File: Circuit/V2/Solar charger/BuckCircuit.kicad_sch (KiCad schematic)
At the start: 2 parts

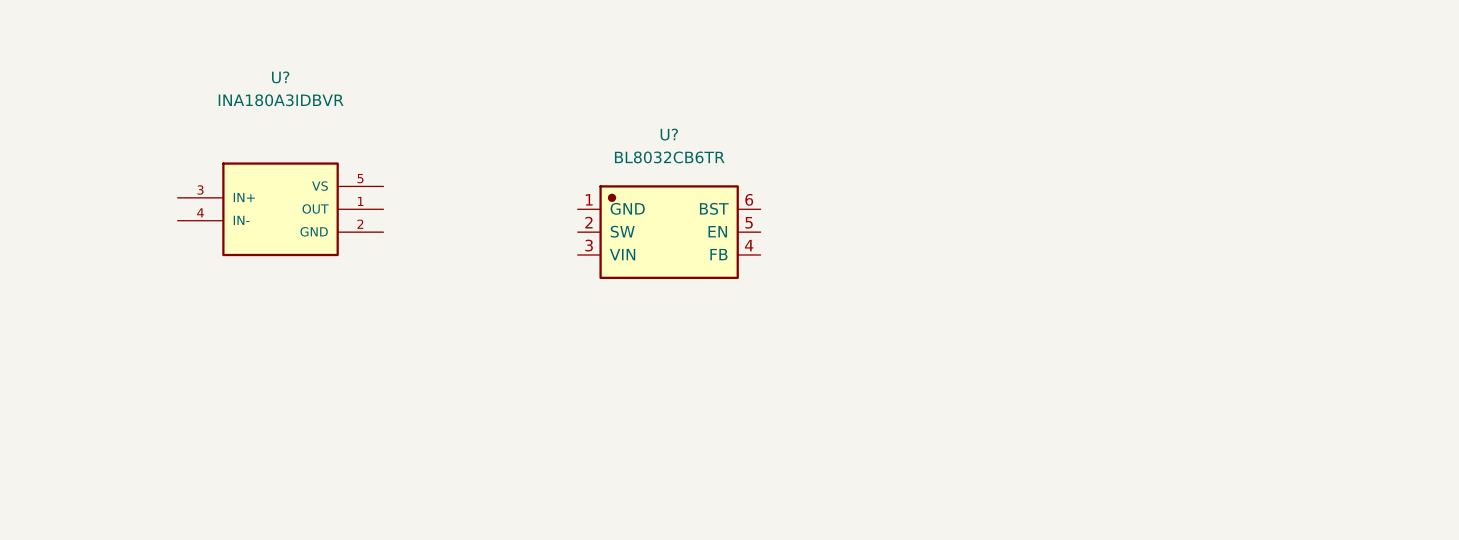
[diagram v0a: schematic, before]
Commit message: update
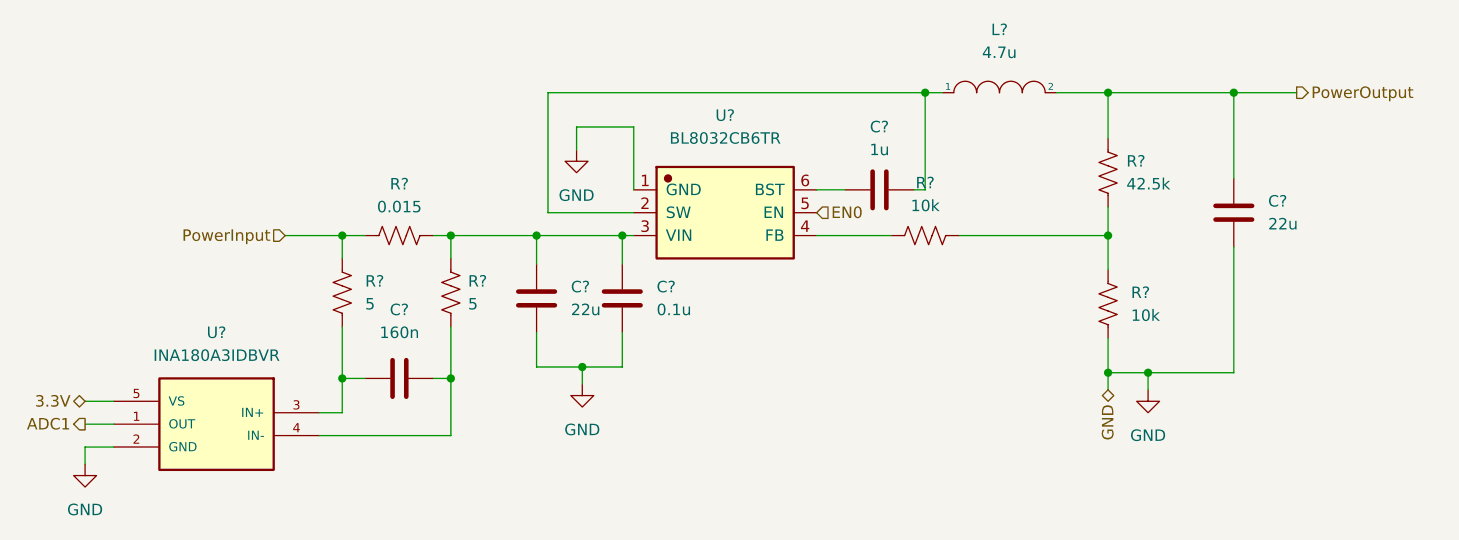
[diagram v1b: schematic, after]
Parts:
- added C?: 1u, Capacitor_SMD:C_0805_2012Metric, symbol 1CommonUse:C0805
- added C? (x2): 22u, Capacitor_SMD:C_0805_2012Metric, symbol 1CommonUse:C0805
- added C?: 0.1u, Capacitor_SMD:C_0805_2012Metric, symbol 1CommonUse:C0805
- added C?: 160n, Capacitor_SMD:C_0805_2012Metric, symbol 1CommonUse:C0805
- added L?: 4.7u, SolarCharger:IND-SMD_L4.5-W4.2, symbol pspice:INDUCTOR
- added R? (x2): 5, Resistor_SMD:R_0805_2012Metric, symbol 1CommonUse:R0805
- added R? (x2): 10k, Resistor_SMD:R_0805_2012Metric, symbol 1CommonUse:R0805
- added R?: 0.015, Resistor_SMD:R_0805_2012Metric, symbol 1CommonUse:R0805
- added R?: 42.5k, Resistor_SMD:R_0805_2012Metric, symbol 1CommonUse:R0805
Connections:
- net ADC1: now reaches U?.1 (OUT)
- net GND: now reaches U?.2 (GND)
- net GND: now also U?.1 (GND), C?.2, C?.2, C?.2, R?.1
- net at U?.3 (IN+): now also C?.1, R?.2
- net at U?.4 (IN-): now also C?.2, R?.1
- net 3.3V: now reaches U?.5 (VS)
- net at U?.2 (SW): now also C?.2, L?.1
- net at U?.3 (VIN): now also C?.1, C?.1, R?.1, R?.2
- net at U?.4 (FB): now also R?.2
- net EN0: now reaches U?.5 (EN)
- net at U?.6 (BST): now also C?.1
- new net: R?.1, R?.1, R?.2
- new net PowerInput: R?.1, R?.2
- new net PowerOutput: C?.1, L?.2, R?.2
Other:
- moved on the sheet: U?
